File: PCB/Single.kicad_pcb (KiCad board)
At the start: 2 copper layers, 317.3 x 143.3 mm, 141 parts, among them SW1 SW_Push, SW10 SW_Push, SW11 SW_Push, SW12 SW_Push, SW13 SW_Push, SW14 SW_Push, SW15 SW_Push, SW16 SW_Push, SW17 SW_Push, SW18 SW_Push, SW19 SW_Push, SW2 SW_Push, SW20 SW_Push, SW21 SW_Push, SW22 SW_Push, SW23 SW_Push, SW24 SW_Push, SW25 SW_Push, SW26 SW_Push, SW27 SW_Push, SW28 SW_Push, SW29 SW_Push, SW3 SW_Push, SW30 SW_Push, SW31 SW_Push, SW32 SW_Push, SW33 SW_Push, SW34 SW_Push, SW35 SW_Push, SW36 SW_Push, SW37 SW_Push, SW38 SW_Push, SW39 SW_Push, SW4 SW_Push, SW40 SW_Push, SW41 SW_Push, SW42 SW_Push, SW43 SW_Push, SW44 SW_Push, SW48 SW_Push, SW49 SW_Push, SW5 SW_Push, SW50 SW_Push, SW51 SW_Push, SW52 SW_Push, SW53 SW_Push, SW54 SW_Push, SW55 SW_Push, SW56 SW_Push, SW57 SW_Push, SW58 SW_Push, SW59 SW_Push, SW6 SW_Push, SW60 SW_Push, SW61 SW_Push, SW62 SW_Push, SW63 SW_Push, SW64 SW_Push, SW7 SW_Push, SW8 SW_Push, SW9 SW_Push, U2 MCP23017_SO, U3 XIAO-nRF52840-SMD

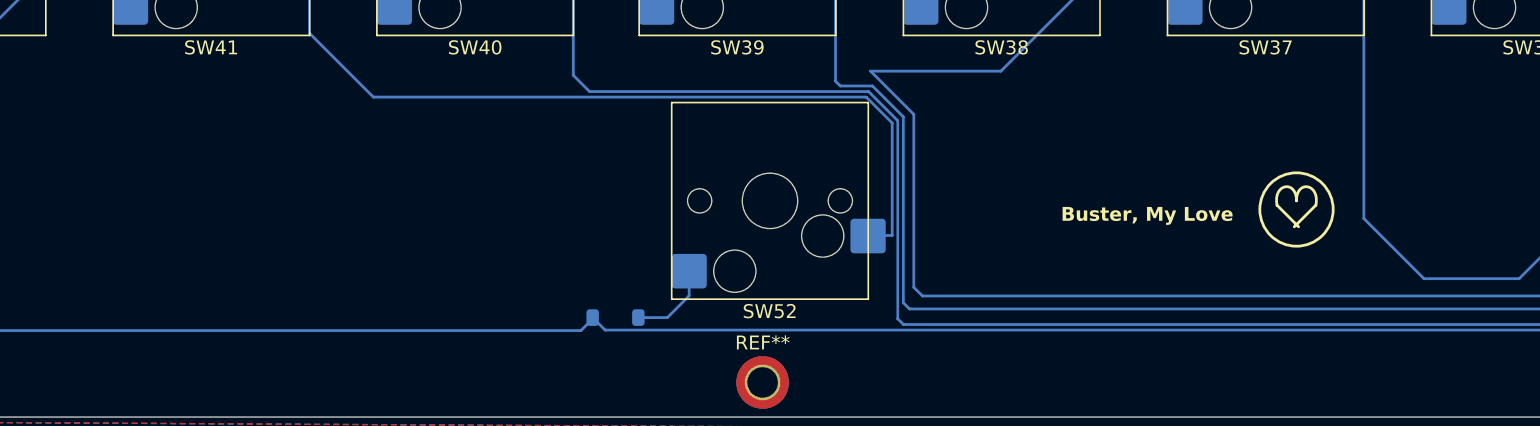
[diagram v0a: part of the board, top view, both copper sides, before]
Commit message: Refactor code structure for improved readability and maintainability
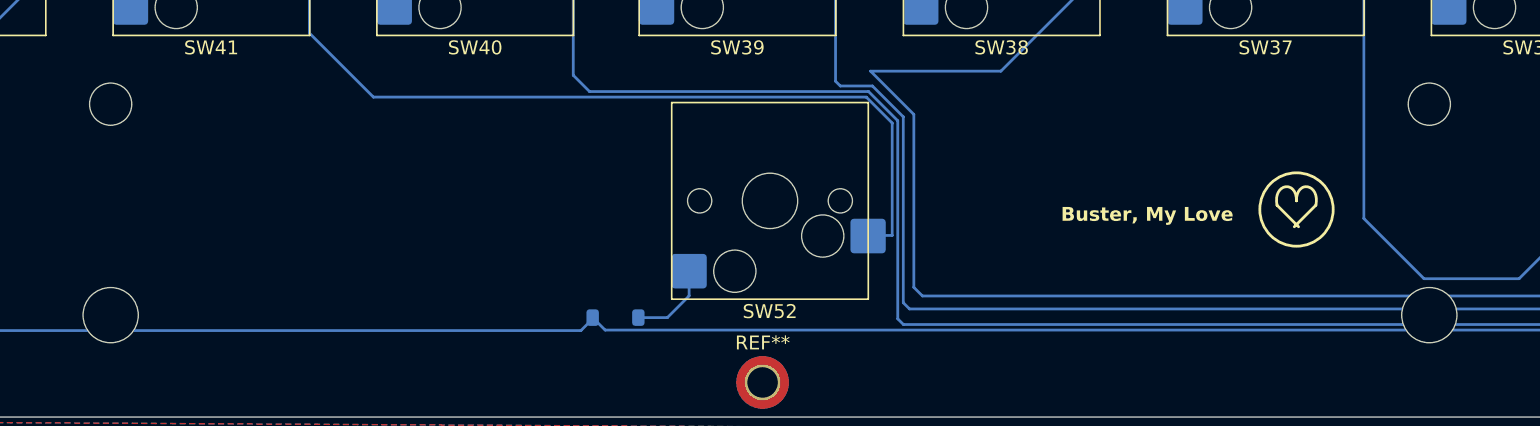
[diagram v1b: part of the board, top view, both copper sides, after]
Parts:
- added REF**: STAB_MX_6u, PCM_marbastlib-mx:STAB_MX_6u, F.Cu at (202.3, 247.6)
